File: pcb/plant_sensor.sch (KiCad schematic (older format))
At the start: 3 parts, among them U1 M95256-WMN6P

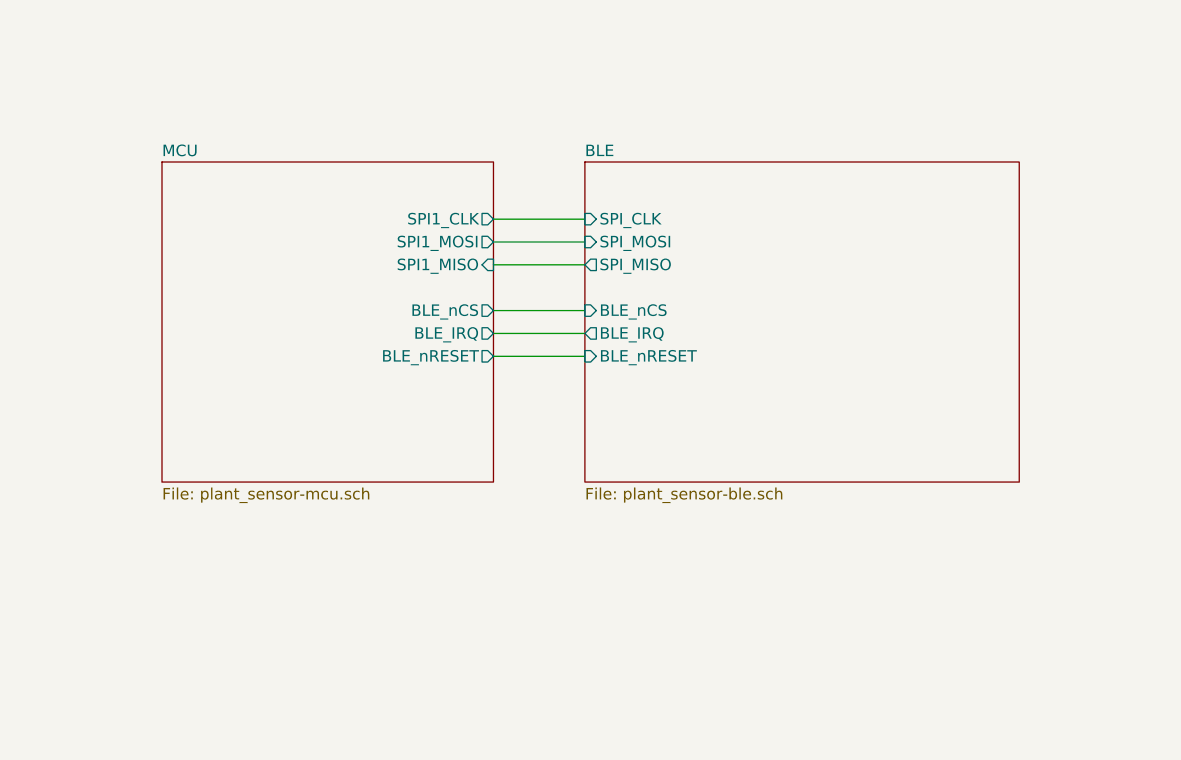
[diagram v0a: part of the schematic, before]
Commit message: Added temperature sensor
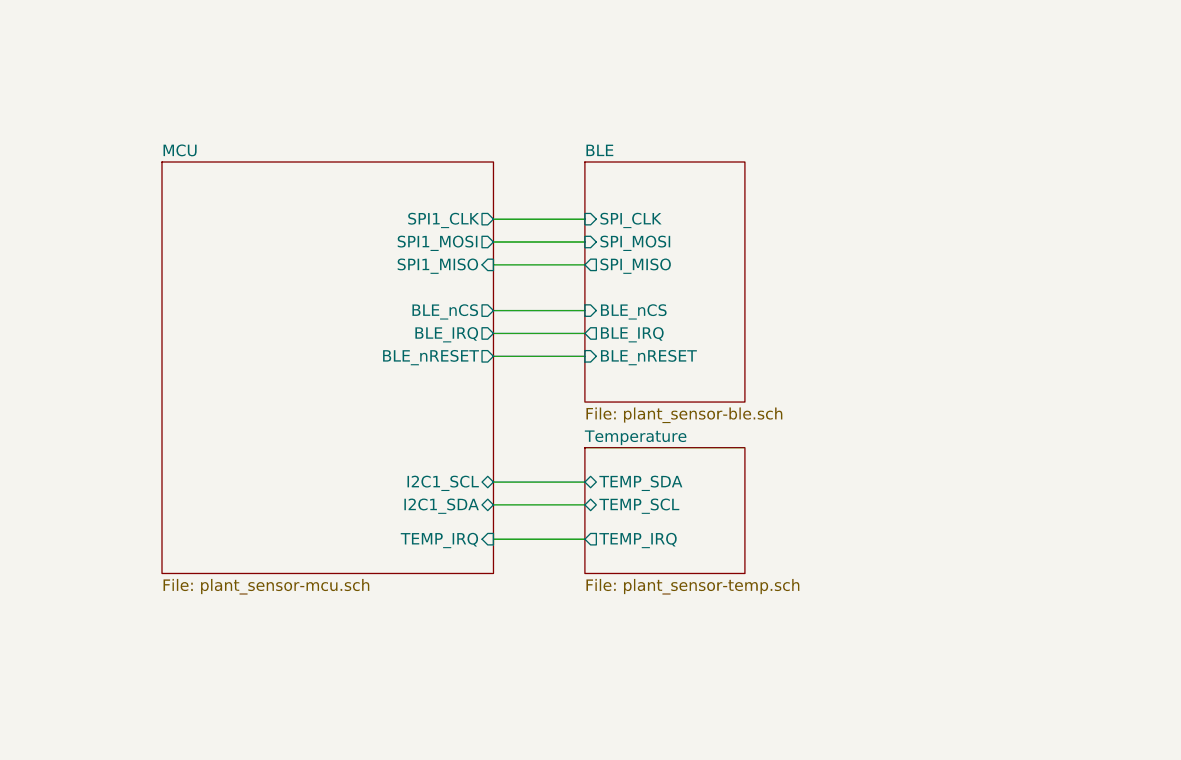
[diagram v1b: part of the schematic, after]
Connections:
- wire segments 14 -> 17
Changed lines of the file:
@@
 EESchema Schematic File Version 4
-LIBS:plant_sensor-cache
 EELAYER 26 0
 EELAYER END
 $Descr A4 11693 8268
 encoding utf-8
-Sheet 1 3
+Sheet 1 4
 Title "Overview"
 Date "2019-02-22"
@@
 $EndDescr
 $Sheet
-S 6700 2500 1900 1400
+S 6700 2500 700  1050
 U 5C6DADA9
 F0 "BLE" 50
@@
 	2150 2200 2150 2300
 $Sheet
-S 4850 2500 1450 1400
+S 4850 2500 1450 1800
 U 5C7262D1
 F0 "MCU" 50
@@
 F6 "BLE_IRQ" O R 6300 3250 50
 F7 "BLE_nRESET" O R 6300 3350 50
+F8 "TEMP_IRQ" I R 6300 4150 50
+F9 "I2C1_SCL" B R 6300 3900 50
+F10 "I2C1_SDA" B R 6300 4000 50
 $EndSheet
 Wire Wire Line
@@
 Wire Wire Line
 	6700 3350 6300 3350
+$Sheet
+S 6700 3750 700  550
+U 5C708F8B
+F0 "Temperature" 50
+F1 "plant_sensor-temp.sch" 50
+F2 "TEMP_SDA" B L 6700 3900 50
+F3 "TEMP_SCL" B L 6700 4000 50
+F4 "TEMP_IRQ" O L 6700 4150 50
+$EndSheet
+Wire Wire Line
+	6300 4000 6700 4000
+Wire Wire Line
+	6700 3900 6300 3900
+Wire Wire Line
+	6300 4150 6700 4150
 $EndSCHEMATC
